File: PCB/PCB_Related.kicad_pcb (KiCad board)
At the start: 4 copper layers, 79.6 x 54.4 mm, 47 parts, among them J1 USB4105-GF-A, Q1 L8050QLT1G, Q2 L8050QLT1G, SW1 SW_Push, SW2 SW_Push, U1 ESP32-C3-WROOM-02U-N4, U2 CP2102N-A02-GQFN28R, U3 AMS1117-3.3

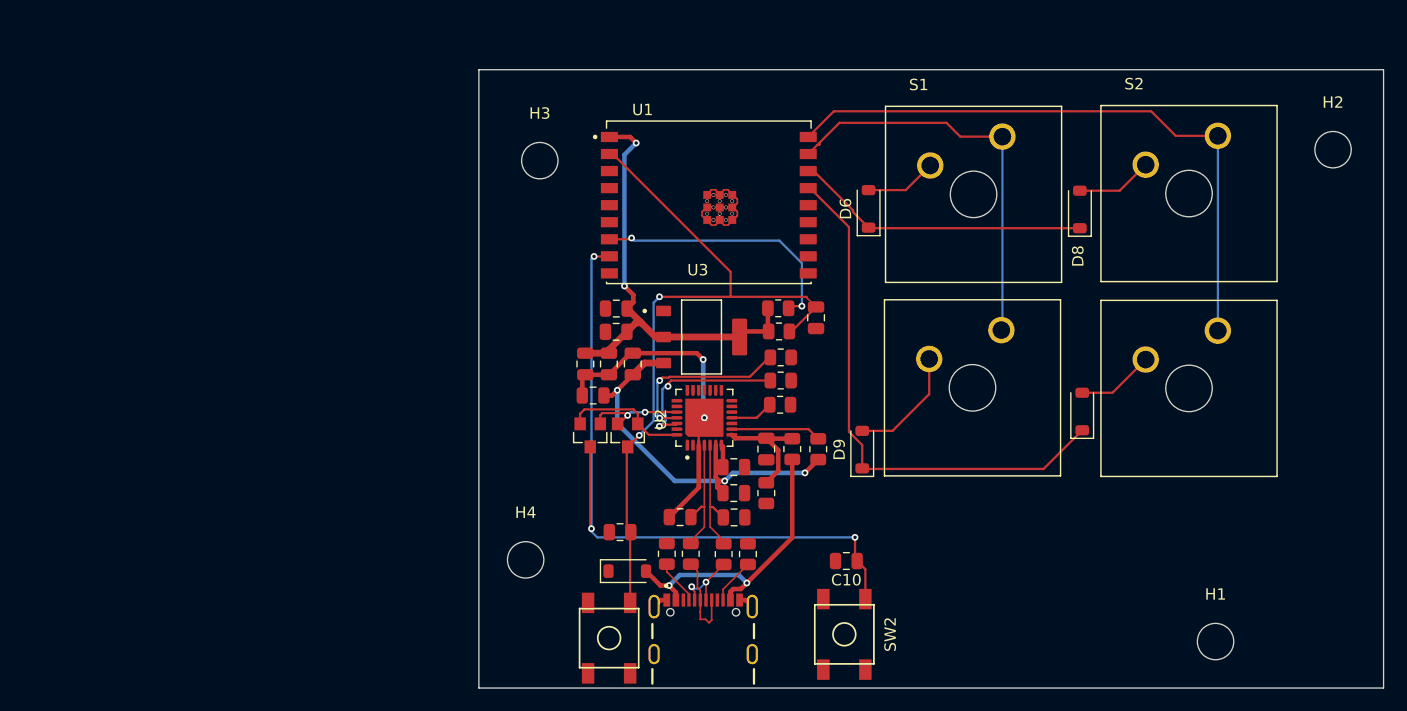
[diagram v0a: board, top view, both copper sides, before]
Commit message: Updated Firmware and Production
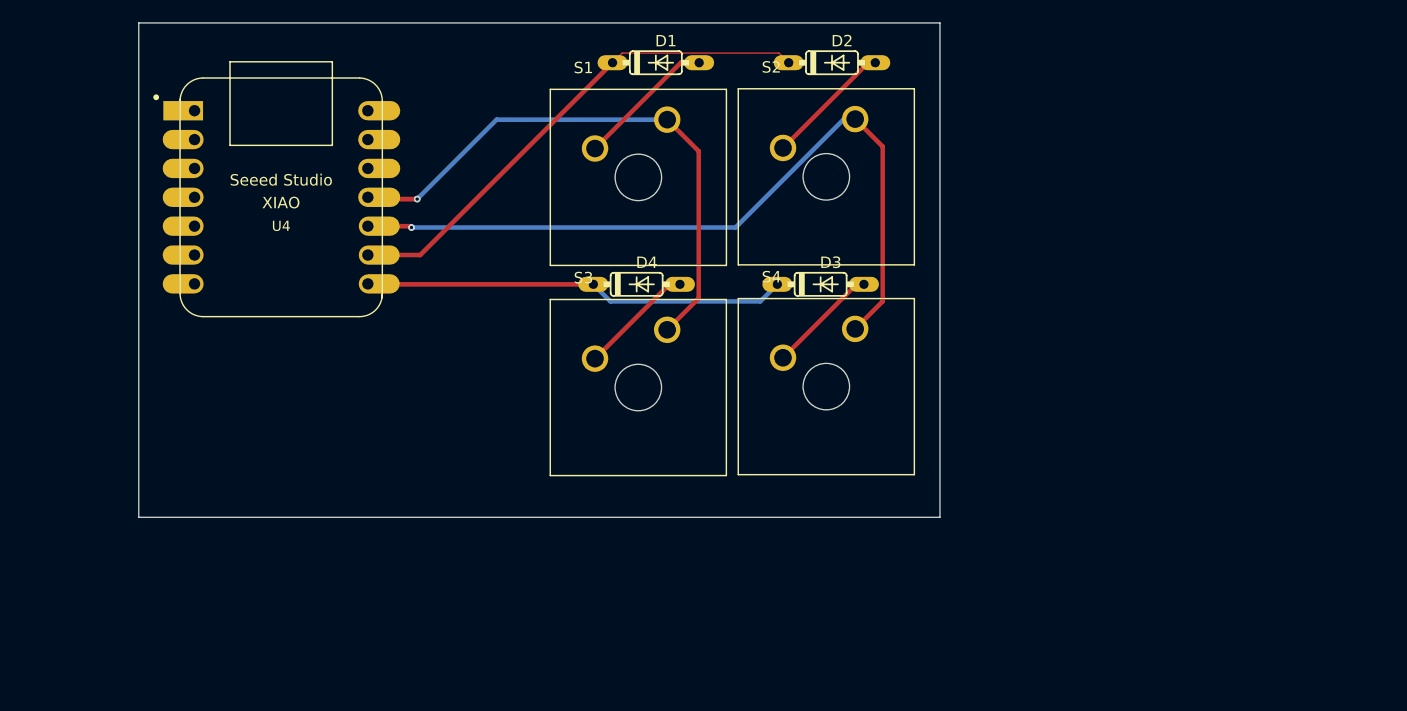
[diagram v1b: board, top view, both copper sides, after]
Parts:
- removed C1, C2: 22pF, Capacitor_SMD:C_0805_2012Metric
- removed C10, C11, C13, C6, C9: 0.1µF/50V, Capacitor_SMD:C_0805_2012Metric
- removed C12, C14, C3, C5, C7: 10µF/25V, Capacitor_SMD:C_0805_2012Metric
- removed C4, C8: 1µF/16V, Capacitor_SMD:C_0805_2012Metric
- removed D10, D6, D8, D9: Z1N5819HW-7-F, Diode_SMD:D_SOD-123
- removed H1, H2, H3, H4: MountingHole, MountingHole:MountingHole_3.2mm_M3
- removed J1: USB4105-GF-A, USB4105-GF-A:GCT_USB4105-GF-A
- removed Q1, Q2: L8050QLT1G, SMD-TRANSISTORS-NPN-25V-500MW_SOT-23_:SOT-23
- removed R1, R2: 51k, Resistor_SMD:R_0805_2012Metric
- removed R10: 1K, Resistor_SMD:R_0805_2012Metric
- removed R11: 22.1K, Resistor_SMD:R_0805_2012Metric
- removed R12: 47.5K, Resistor_SMD:R_0805_2012Metric
- removed R13, R14, R7, R8: 0, Resistor_SMD:R_0805_2012Metric
- removed R15, R16, R9: 10K, Resistor_SMD:R_0805_2012Metric
- removed SW1, SW2: SW_Push, random-keyboard-parts:SKQG-1155865
- removed U1: ESP32-C3-WROOM-02U-N4, ESP32-C3-WROOM-02U-N4:XCVR_ESP32-C3-WROOM-02U-N4
- removed U2: CP2102N-A02-GQFN28R, CP2102N-A02-GQFN28R:IC_CP2102N-A02-GQFN28R
- removed U3: AMS1117-3.3, AMS1117-3.3:SOT229P700X180-4N
- added D1: 1N4148, 1N4148:DO35-7, F.Cu at (109.5, 21.0)
- added D2: 1N4148, 1N4148:DO35-7, F.Cu at (125.0, 21.0)
- added D4: 1N4148, 1N4148:DO35-7, F.Cu at (107.8, 40.5)
- added U4: MOUDLE-SEEEDUINO-XIAO, XIAO_RP2040:XIAO-Generic-Hybrid-14P-2.54-21X17.8MM, F.Cu at (76.5, 32.8)
- D3: value LESD5D5.0CT1G -> 1N4148; footprint Diode_SMD:D_SOD-123 -> 1N4148:DO35-7
- moved S2 31.9 mm to (124.5, 31.0)
- moved S4 31.9 mm to (124.5, 49.5)
- moved D3 30.4 mm to (124.0, 40.5)
- moved S1 29.5 mm to (108.0, 31.1)
- moved S3 29.4 mm to (108.0, 49.6)
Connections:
- S4 pad 1: Net-(D10-A) -> Net-(D3-PadA)
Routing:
- net +3V3: track 77.3 -> 0.00 mm, vias 5 -> 0
- net CHIP_PU: track 62.9 -> 0.00 mm, vias 2 -> 0
- net GPIO9: track 62.1 -> 0.00 mm, vias 3 -> 0
- net GND: track 45.3 -> 0.00 mm, vias 2 -> 0
- net VBUS: track 26.6 -> 0.00 mm, vias 2 -> 0
- net GPIO8: track 22.9 -> 0.00 mm, vias 2 -> 0
- net ROW0: track 26.1 -> 44.3 mm
- net Net-(U2-RXD): track 15.6 -> 0.00 mm, vias 2 -> 0
- net Net-(U2-TXD): track 15.3 -> 0.00 mm, vias 2 -> 0
- net COL0: track 35.9 -> 49.6 mm, vias 0 -> 1
- net COL1: track 55.0 -> 66.9 mm, vias 0 -> 1
- net DTR: track 11.0 -> 0.00 mm
- net ROW1: track 47.5 -> 36.8 mm
- net USB_DP: track 10.5 -> 0.00 mm
- net USB_DN: track 10.4 -> 0.00 mm
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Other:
- board size 79.6 x 54.4 mm -> 70.5 x 43.5 mm

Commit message: Updated Final version V1
Updated the pcb, schematic, cad, and code. Update the gerbers
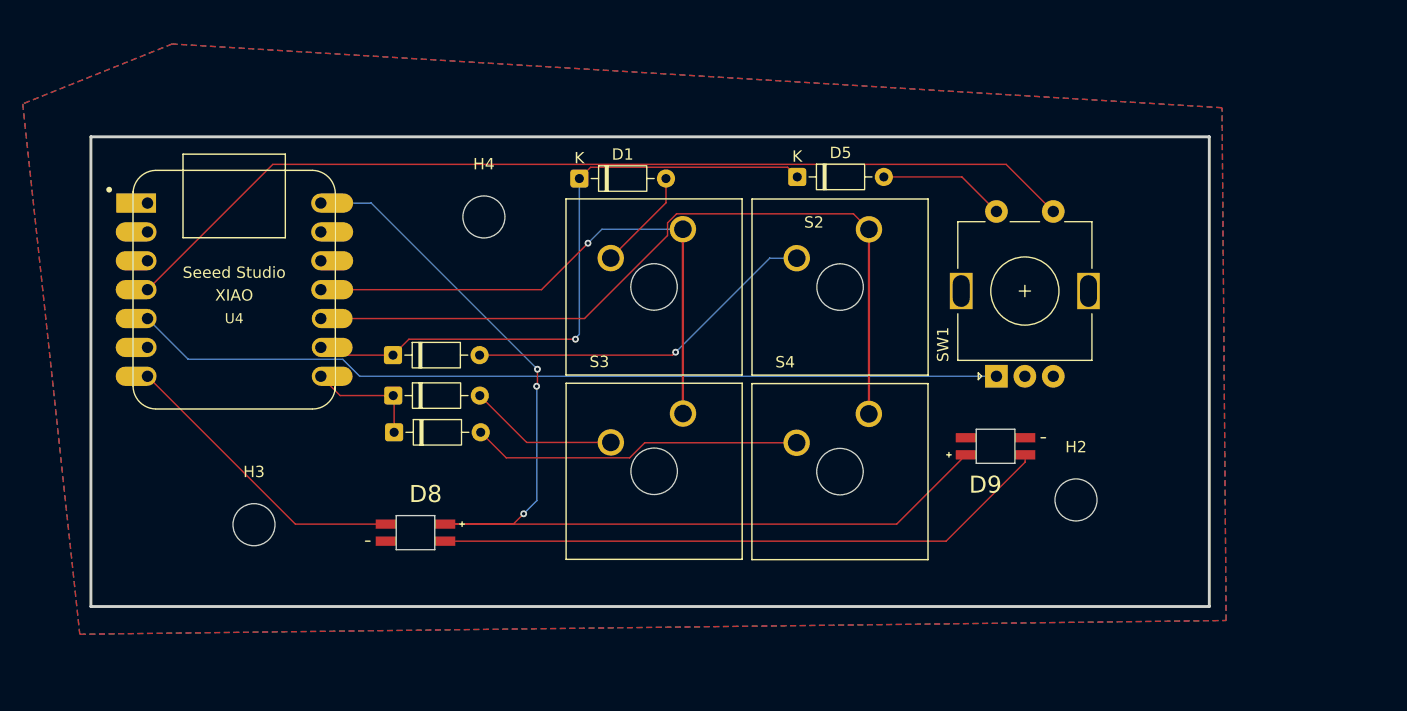
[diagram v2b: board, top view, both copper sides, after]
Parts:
- added D5: D_Small, Diode_THT:D_DO-35_SOD27_P7.62mm_Horizontal, F.Cu at (121.9, 31.1)
- added D8: SK6812-E, SK6812-E:LED_SK6812-E, F.Cu at (88.3, 62.4)
- added D9: SK6812-E, SK6812-E:LED_SK6812-E, F.Cu at (139.4, 54.8)
- added H2: MountingHole, MountingHole:MountingHole_3.7mm, F.Cu at (146.5, 59.5)
- added H3: MountingHole, MountingHole:MountingHole_3.7mm, F.Cu at (74.1, 61.6)
- added H4: MountingHole, MountingHole:MountingHole_3.7mm, F.Cu at (94.4, 34.6)
- added SW1: RotaryEncoder_Switch, Rotary_Encoder:RotaryEncoder_Alps_EC11E-Switch_Vertical_H20mm, F.Cu at (139.5, 48.6)
- D1, D2, D3, D4: value 1N4148 -> D_Small; footprint 1N4148:DO35-7 -> Diode_THT:D_DO-35_SOD27_P7.62mm_Horizontal
- moved D2 46.4 mm to (86.4, 46.7)
- moved D3 38.9 mm to (86.4, 50.3)
- moved D4 25.0 mm to (86.5, 53.5)
- moved D1 12.2 mm to (102.8, 31.2)
- moved S2 9.78 mm to (125.7, 40.7)
- moved S1 9.74 mm to (109.3, 40.7)
- moved U4 9.12 mm to (72.4, 41.0)
- moved S4 7.58 mm to (125.7, 57.0)
- moved S3 7.50 mm to (109.3, 57.0)
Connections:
- S1 pad 1: Net-(D1-PadA) -> Net-(D1-A)
- S2 pad 1: Net-(D2-PadA) -> Net-(D2-A)
- S3 pad 1: Net-(D4-PadA) -> Net-(D3-A)
- S4 pad 1: Net-(D3-PadA) -> Net-(D4-A)
- U4 pad 14: unconnected-(U4-5V-Pad14) -> VCC
- U4 pad 4: unconnected-(U4-PA11_A3_D3-Pad4) -> B
- U4 pad 5: unconnected-(U4-PA8_A4_D4_SDA-Pad5) -> AUP
- U4 pad 6: unconnected-(U4-PA9_A5_D5_SCL-Pad6) -> BDOWN
- U4 pad 7: unconnected-(U4-PB08_A6_D6_TX-Pad7) -> LED
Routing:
- net VCC: track 0.00 -> 94.0 mm, vias 0 -> 3
- net B: track 0.00 -> 86.0 mm
- net AUP: track 0.00 -> 76.8 mm
- net Net-(D8-DOUT): track 0.00 -> 54.6 mm
- net Net-(D2-A): track 0.00 -> 31.4 mm, vias 0 -> 1
- net Net-(D4-A): track 0.00 -> 29.3 mm
- net ROW1: track 36.8 -> 10.3 mm
- net LED: track 0.00 -> 26.4 mm
- net Net-(D3-A): track 0.00 -> 13.2 mm
- net ROW0: track 44.3 -> 57.5 mm, vias 0 -> 1
- net Net-(D1-PadA): track 12.3 -> 0.00 mm
- net Net-(D2-PadA): track 11.2 -> 0.00 mm
- net A: track 0.00 -> 11.2 mm
- net Net-(D4-PadA): track 10.2 -> 0.00 mm
- net Net-(D3-PadA): track 9.80 -> 0.00 mm
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- added copper zone on B.Cu, net GND
- added copper zone on F.Cu, net GND
- added copper zone on In1.Cu, net GND
- added copper zone on In2.Cu, net GND
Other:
- board size 70.5 x 43.5 mm -> 98.4 x 41.3 mm
